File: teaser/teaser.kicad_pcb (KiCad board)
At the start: 2 copper layers, 43 x 136 mm, 71 parts, among them J1 Programator, J2 AC_Plug, J3 OLED, J4 battery, Q1 MMBTA44, Q2 MMBTA44, Q3 MMBTA44, Q4 MMBTA44, Q6 AO3401A, SW1 Włancznik, SW2 SW_SPST, SW3 Manual, SW4 Manual, SW5 Manual, SW7 SW_Push, U2 LM1117MP-5.0, U3 ATmega328P-A, Y1 16kHz

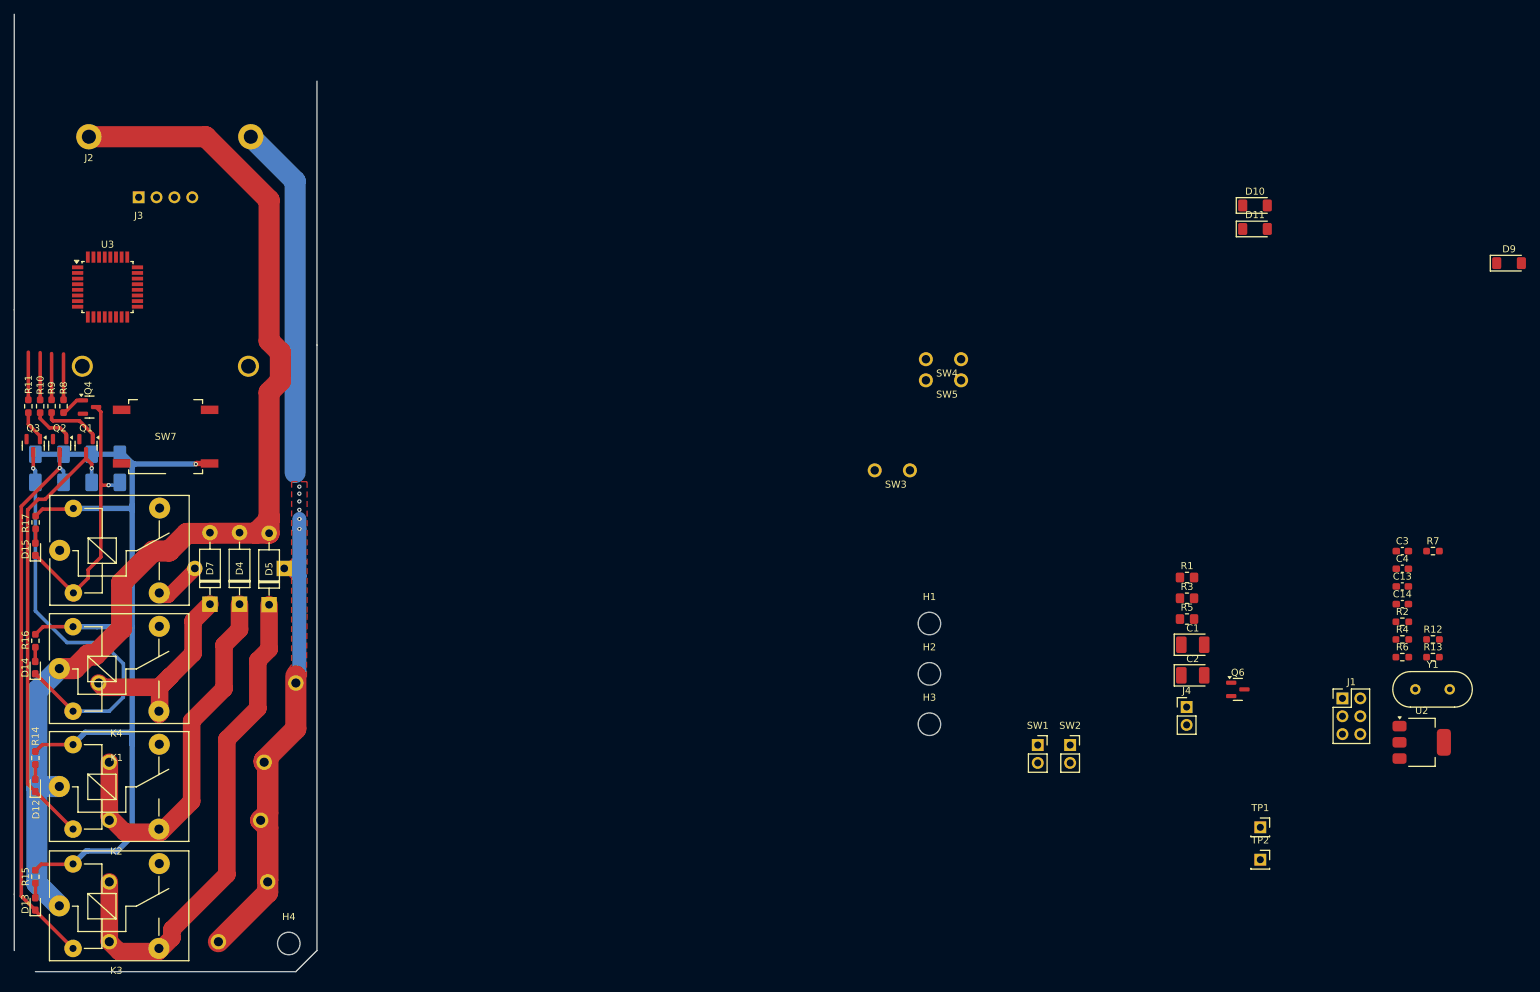
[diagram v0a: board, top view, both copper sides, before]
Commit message: Continue routing
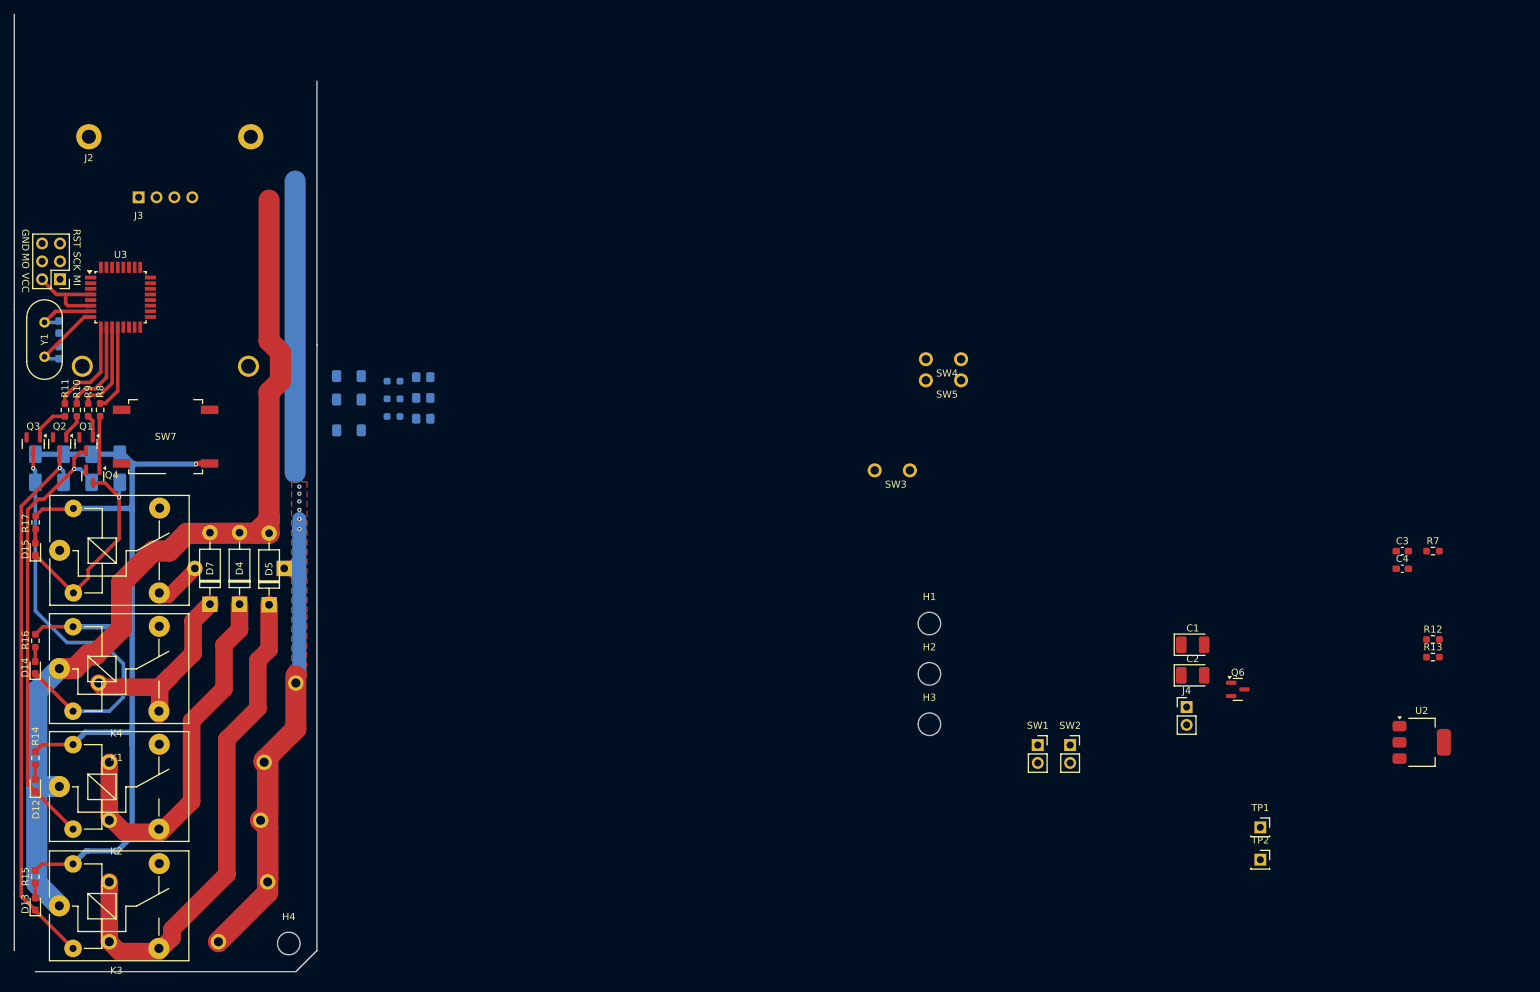
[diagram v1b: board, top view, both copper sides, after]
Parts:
- C13, C14, D10, D11, D9, R1, R2, R3, R4, R5, R6: moved to B.Cu
- moved Y1 200.4 mm to (55.3, 93.7), turned to 90 degrees
- moved C13 194.4 mm to (57.3, 89.4), turned to 90 degrees
- moved C14 194.2 mm to (57.3, 93.1), turned to -90 degrees
- moved J1 191.7 mm to (57.5, 82.6), turned to 180 degrees
- moved D9 166.5 mm to (98.5, 104.1), turned to 180 degrees
- moved R2 147.3 mm to (104.9, 97.1), turned to 180 degrees
- moved R4 147.3 mm to (104.9, 99.6), turned to 180 degrees
- moved R6 147.3 mm to (104.9, 102.1), turned to 180 degrees
- moved D10 131.0 mm to (98.5, 96.4), turned to 180 degrees
- moved D11 131.0 mm to (98.5, 99.7), turned to 180 degrees
- moved R1 112.2 mm to (109.1, 96.5), turned to 180 degrees
- moved R3 112.2 mm to (109.1, 99.5), turned to 180 degrees
- moved R5 112.2 mm to (109.1, 102.5), turned to 180 degrees
- moved Q4 9.85 mm to (62.1, 110.6), turned to -90 degrees
- moved R10 5.23 mm to (59.9, 101.2)
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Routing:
- net Net-(D2-K): track 139.1 -> 88.8 mm
- net GND: track 0.00 -> 41.4 mm
- net Net-(D4-A): track 162.0 -> 132.7 mm
- net VCC: track 139.5 -> 152.3 mm
- net Net-(U3-XTAL2/PB7): track 0.00 -> 11.0 mm
- net Net-(U3-XTAL1/PB6): track 0.00 -> 9.28 mm
- net Net-(D1-A): track 38.8 -> 30.6 mm
- net /CH1: track 6.78 -> 13.9 mm
- net /CH2: track 6.71 -> 13.4 mm
- net /CH3: track 6.56 -> 13.0 mm
- net /MEASURE_EN: track 6.51 -> 12.3 mm
- net Net-(Q1-B): track 8.38 -> 3.26 mm
- net Net-(Q4-B): track 3.47 -> 7.63 mm
- net Net-(Q2-B): track 6.17 -> 3.59 mm
- net Net-(Q3-B): track 4.43 -> 5.46 mm
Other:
- board text added: "GND"
- board text added: "MI"
- board text added: "MO"
- board text added: "RST"
- board text added: "SCK"
- board text added: "VCC"
